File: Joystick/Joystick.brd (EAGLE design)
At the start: 36.3 x 29.8 mm, 11 parts

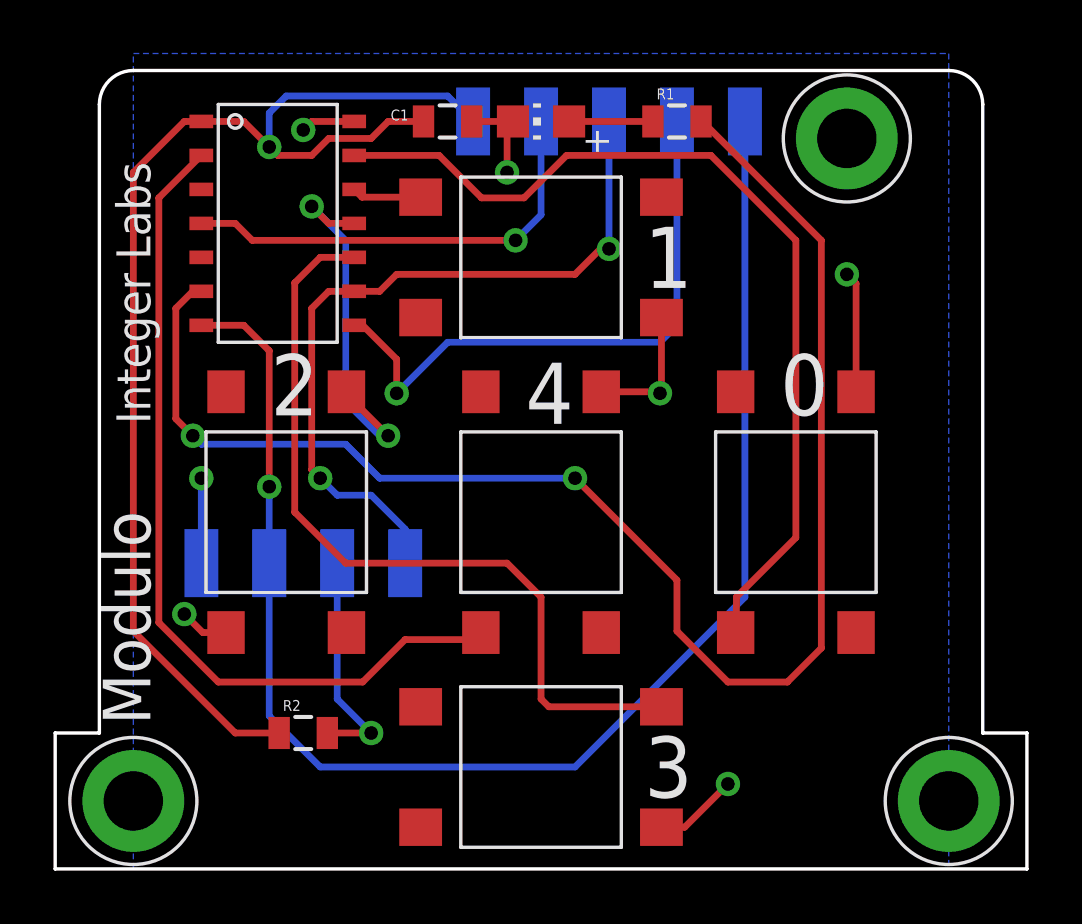
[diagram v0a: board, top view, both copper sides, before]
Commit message: Checkpointing PCB designs
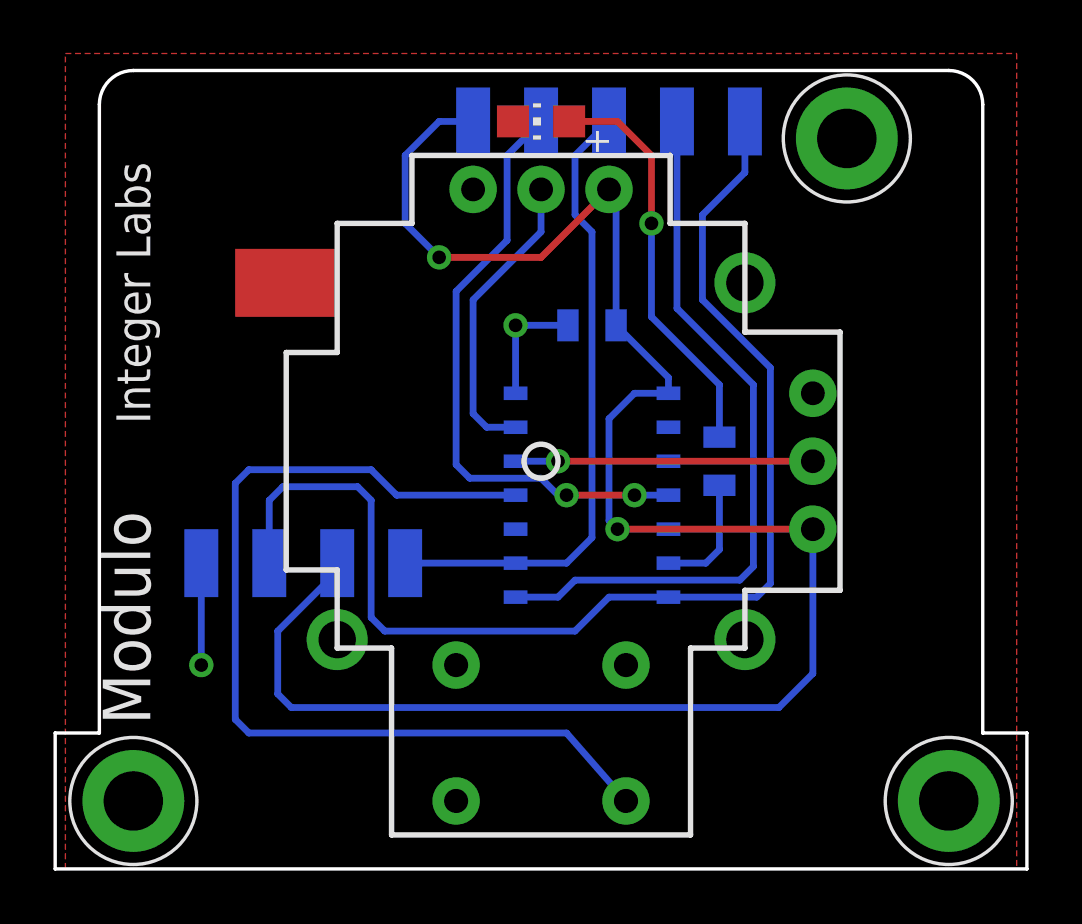
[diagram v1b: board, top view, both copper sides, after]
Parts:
- removed B1, B3, B4, B5, B7: TACT-SWITCH, IntegerLabs:MJTP1138
- removed R1: 680, SparkFun-Passives:0805
- added U1: JOYSTICKPTH, IntegerLabs:JOYSTICK
- R2: value 1 -> 680; device SparkFun-Resistors:0805 -> SparkFun-Passives:0805
- moved R2 18.6 mm to (24.4, 15.2), flipped to the bottom, turned to 270 degrees
- moved U$1 15.1 mm to (19.4, 17.8), flipped to the bottom
- moved C1 9.34 mm to (19.7, 20.3), flipped to the bottom
- renumbered U$2 to U$7
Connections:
- removed net BUTTON0: B5.POS1, U$1.13
- removed net BUTTON1: B1.POS1, U$1.12
- removed net BUTTON2: B3.POS1, U$1.11
- removed net BUTTON3: B7.POS2, U$1.10
- removed net BUTTON4: B4.POS1, U$1.2
- removed net N$2: R2.2, U$7.BUS2
- removed net N$8: LED1.A, R1.1
- new net H: U$1.13, U1.H2
- new net N$7: LED1.A, R2.1
- new net SEL: U$1.11, U1.B1A
- new net V: U$1.12, U1.V2
- net GND: now also U1.B2A, U1.H3, U1.V3; no longer B1.NEG2, B3.NEG2, B4.NEG2, B5.NEG2, B7.NEG2
- net LED: now also R2.2; no longer R1.2
- net VCC: now also U$7.BUS2, U1.H1, U1.V1; no longer R2.1
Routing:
- net LED: track 56.8 -> 4.52 mm, vias 2 -> 0
- net SEL: track 0.00 -> 35.9 mm
- net BUTTON0: track 34.7 -> 0.00 mm
- net BUTTON4: track 31.8 -> 0.00 mm
- net BUTTON3: track 30.1 -> 0.00 mm
- net VCC: track 46.4 -> 69.5 mm, vias 1 -> 2
- net N$7: track 0.00 -> 15.2 mm, vias 0 -> 1
- net GND: track 23.4 -> 8.31 mm, vias 7 -> 2
- net BUTTON2: track 14.1 -> 0.00 mm, vias 2 -> 0
- net H: track 0.00 -> 11.2 mm
- net V: track 0.00 -> 11.1 mm, vias 0 -> 1
- net SDA/MOSI: track 55.6 -> 45.8 mm, vias 1 -> 0
- net N$2: track 8.52 -> 0.00 mm, vias 1 -> 0
- net RESET: track 16.9 -> 22.6 mm, vias 1 -> 2
- net SCL/SCK: track 28.5 -> 23.7 mm, vias 2 -> 0
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- added copper zone on layer 1, net GND
- removed copper zone on layer 16, net GND
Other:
- board text removed: "0"
- board text removed: "1"
- board text removed: "2"
- board text removed: "3"
- board text removed: "4"
